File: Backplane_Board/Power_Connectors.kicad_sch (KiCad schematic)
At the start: 15 parts, among them J1 Conn_01x02_Pin, J10 Conn_01x02_Pin, J11 Conn_01x02_Pin, J12 Conn_01x02_Pin, J13 Conn_01x02_Pin, J14 Conn_01x02_Pin, J15 Conn_01x02_Pin, J16 Conn_01x02_Pin, J2 Conn_01x02_Pin, J4 Conn_01x02_Pin, J5 Conn_01x02_Pin, J6 Conn_01x02_Pin, J7 Conn_01x02_Pin, J8 Conn_01x02_Pin, J9 Conn_01x02_Pin

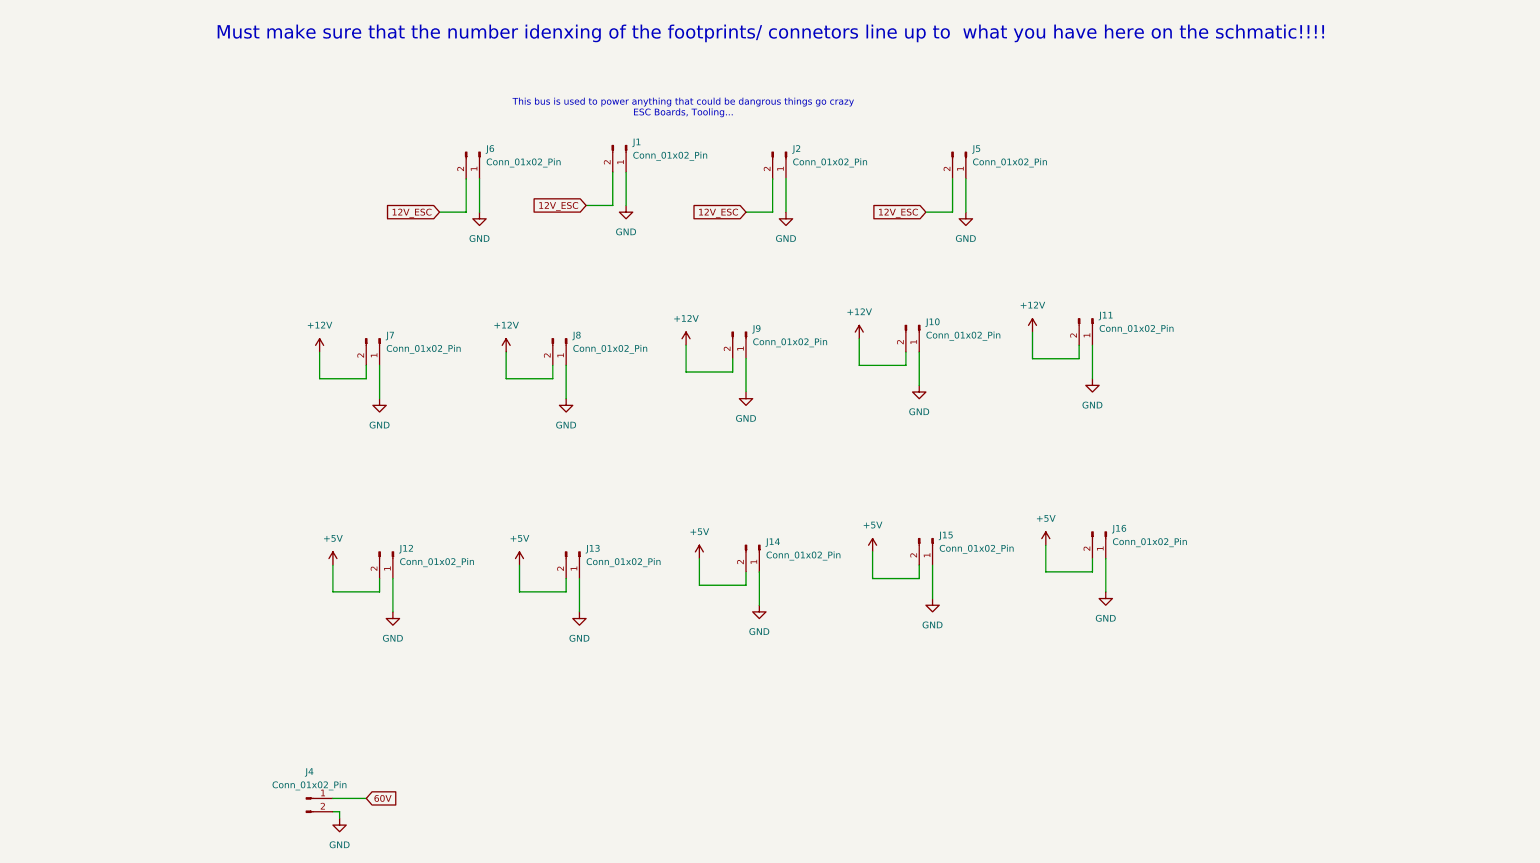
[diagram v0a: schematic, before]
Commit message: back plane board ready for review
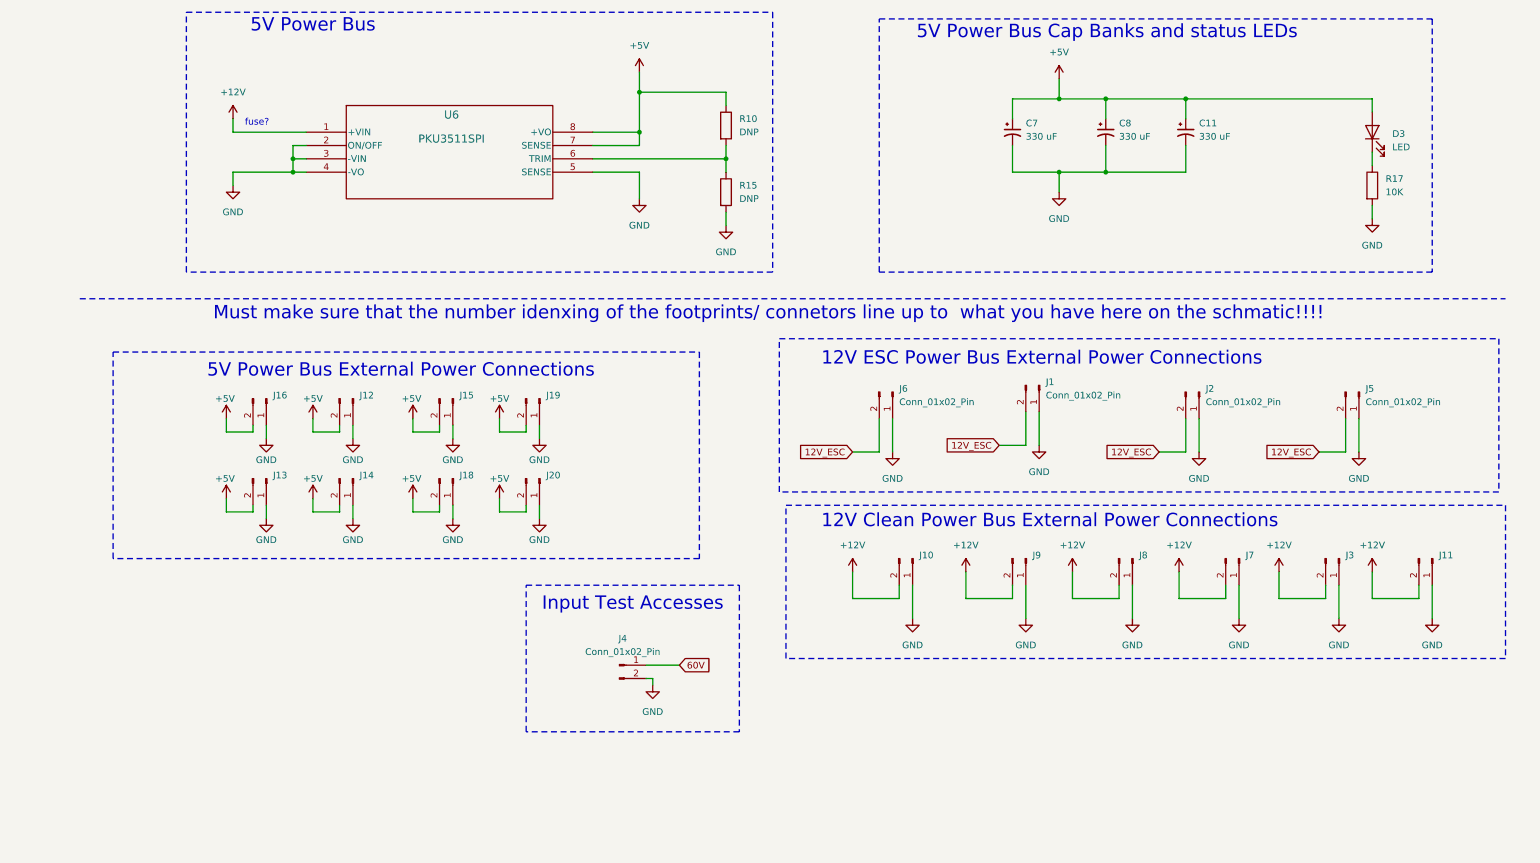
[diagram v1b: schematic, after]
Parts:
- added C11, C7, C8: 330 uF, 220UF CAP:CAP_16SVPG330MX, symbol Device:C_Polarized_Small_US
- added D3: LED, symbol Device:LED
- added J18, J19, J20, J3: Conn_01x02_Pin, symbol Connector:Conn_01x02_Pin
- added R10, R15: DNP, symbol Device:R
- added R17: 10K, symbol Device:R
- added U6: PKU3511SPI, PKU 3500S_FPM, symbol PKU3511SPI:PKU3511SPI
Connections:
- net +12V: now also J3.2 (Pin_2), U6.1 (+VIN)
- net +5V: now also C11.1, C7.1, C8.1, D3.2 (A), J18.2 (Pin_2), J19.2 (Pin_2), J20.2 (Pin_2), R10.1, U6.7 (SENSE), U6.8 (+VO)
- net GND: now also C11.2, C7.2, C8.2, J18.1 (Pin_1), J19.1 (Pin_1), J20.1 (Pin_1), J3.1 (Pin_1), R15.2, R17.2, U6.2 (ON/OFF), U6.3 (-VIN), U6.4 (-VO), U6.5 (SENSE)
- new net: R10.2, R15.1, U6.6 (TRIM)
- new net: D3.1 (K), R17.1
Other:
- note added: "12V Clean Power Bus External Power Connections"
- note added: "12V ESC Power Bus External Power Connections"
- note added: "5V Power Bus"
- note added: "5V Power Bus Cap Banks and status LEDs"
- note added: "5V Power Bus External Power Connections"
- note added: "Input Test Accesses"
- note added: "fuse?"
- note removed: "This bus is used to power anything that could be dangrous things go crazy ESC Boards, Tooling..."
- moved on the sheet: J1, J11, J16, J2, J4, J5, J6
